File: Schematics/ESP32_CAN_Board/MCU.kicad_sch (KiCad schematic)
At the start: 13 parts, among them J1 Screw_Terminal_01x04, J2 Screw_Terminal_01x04, J3 Screw_Terminal_01x02, U4 ESP32-C3-MINI-1-N4

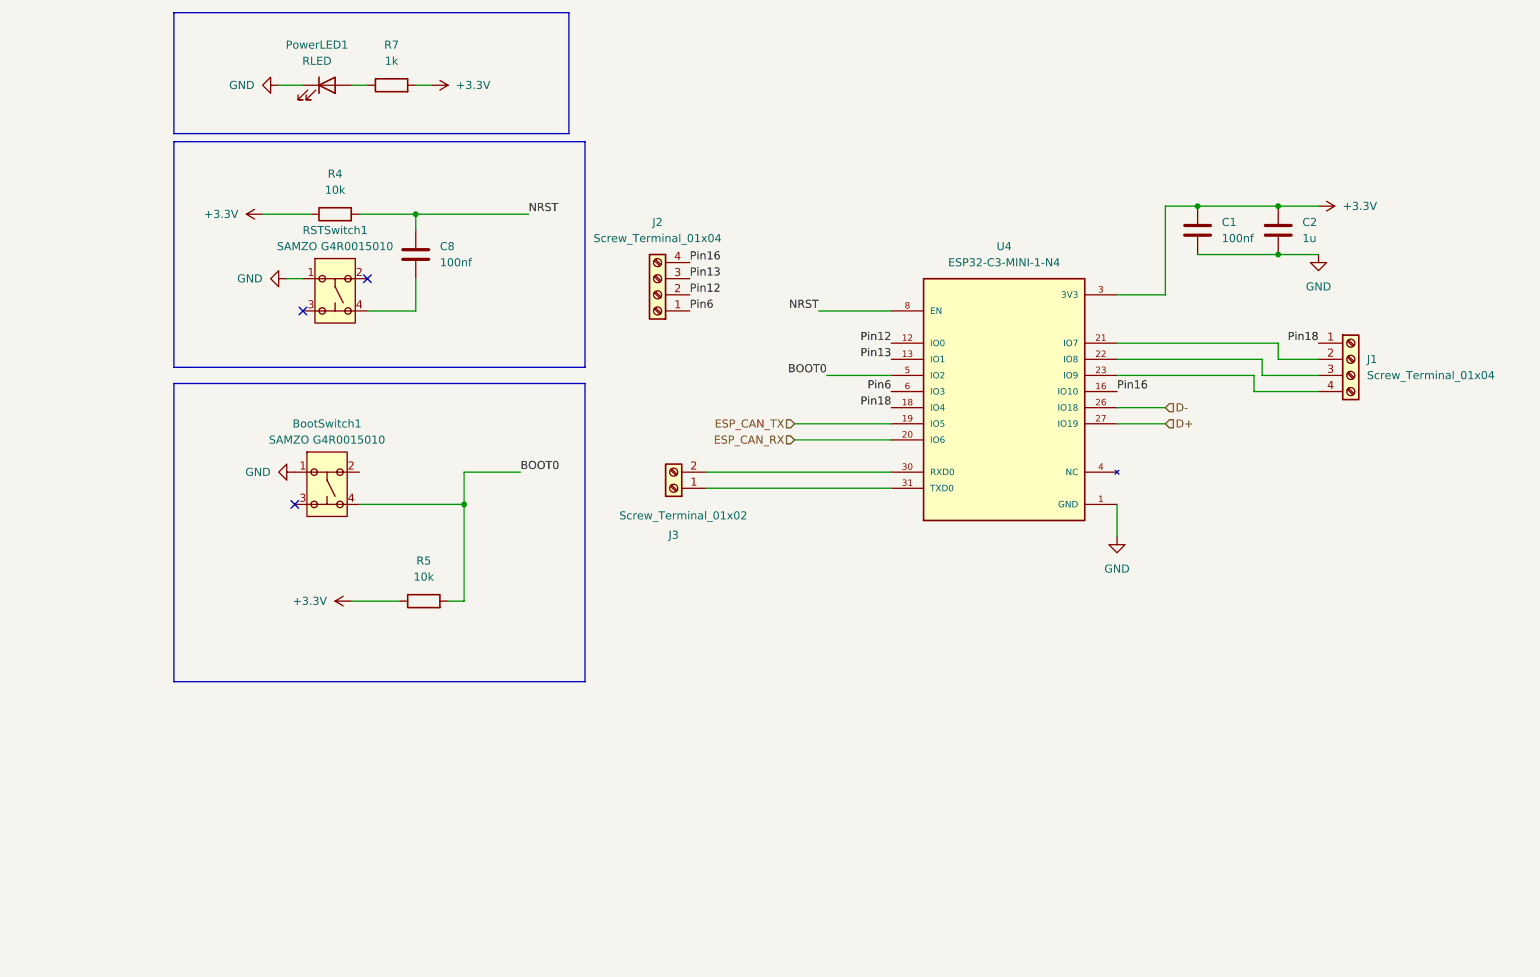
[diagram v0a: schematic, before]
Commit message: updated ESPBoard
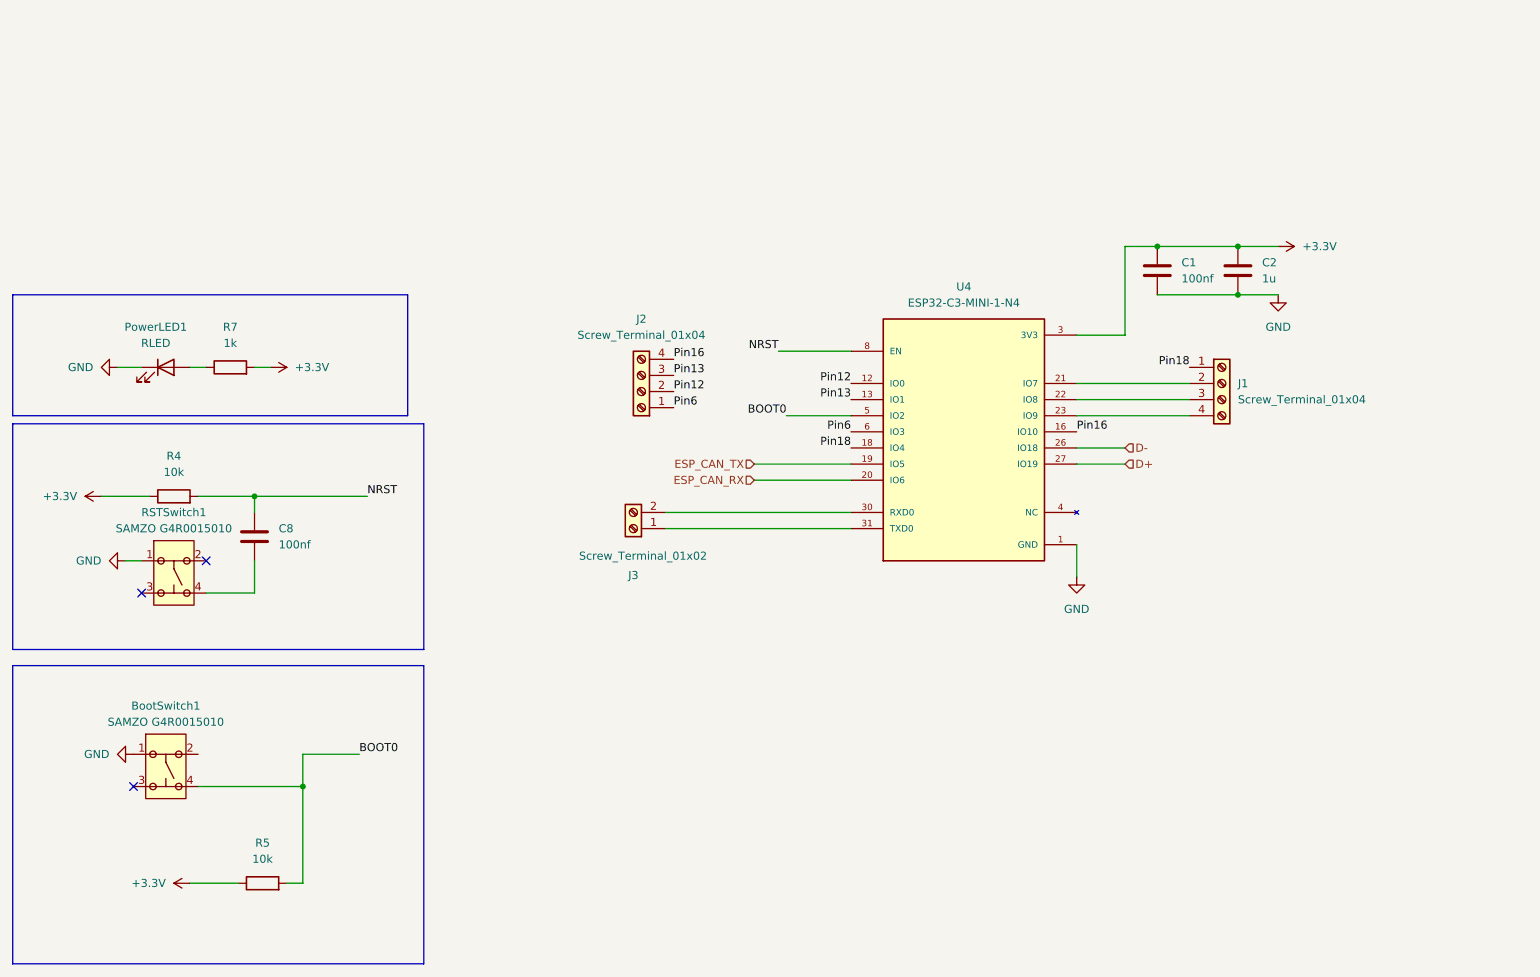
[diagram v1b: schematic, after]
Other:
- moved on the sheet: BootSwitch1, C1, C2, C8, J1, J2, J3, PowerLED1, R4, R5, R7, RSTSwitch1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
